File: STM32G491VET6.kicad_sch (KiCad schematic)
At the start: 37 parts, among them CN3 C2839705, CN4 C2839704, J2 TC2030, U2 TYPE-C 16PLT-H10.0, U3 STM32G431CBT6, U9 TCAN3403DRQ1, X1 NX3215SA 32.768KHZ EXS00A-MU0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, X2 NDK NX2016SA-24MHZ-EXS00A-CS1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

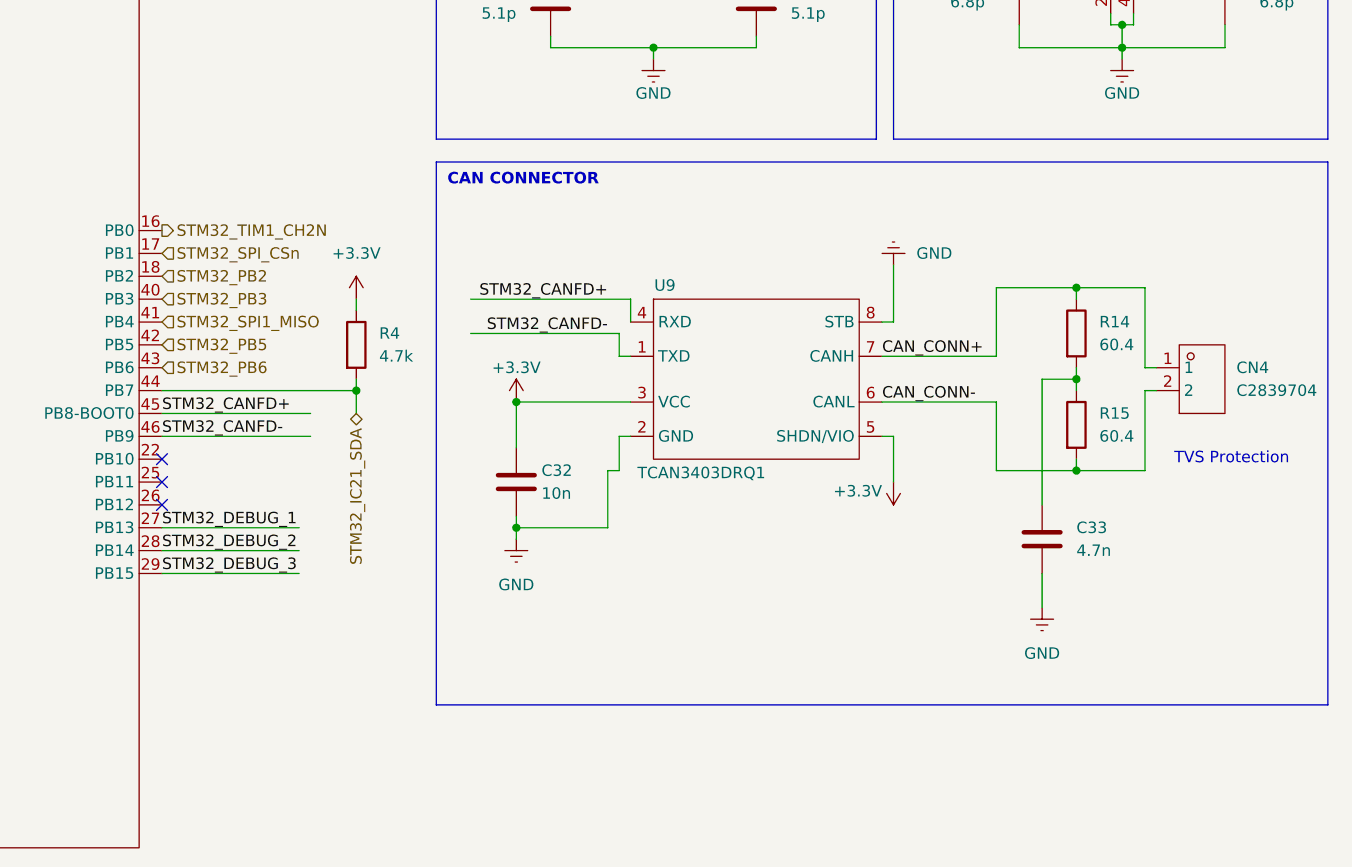
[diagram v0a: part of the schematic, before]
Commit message: update
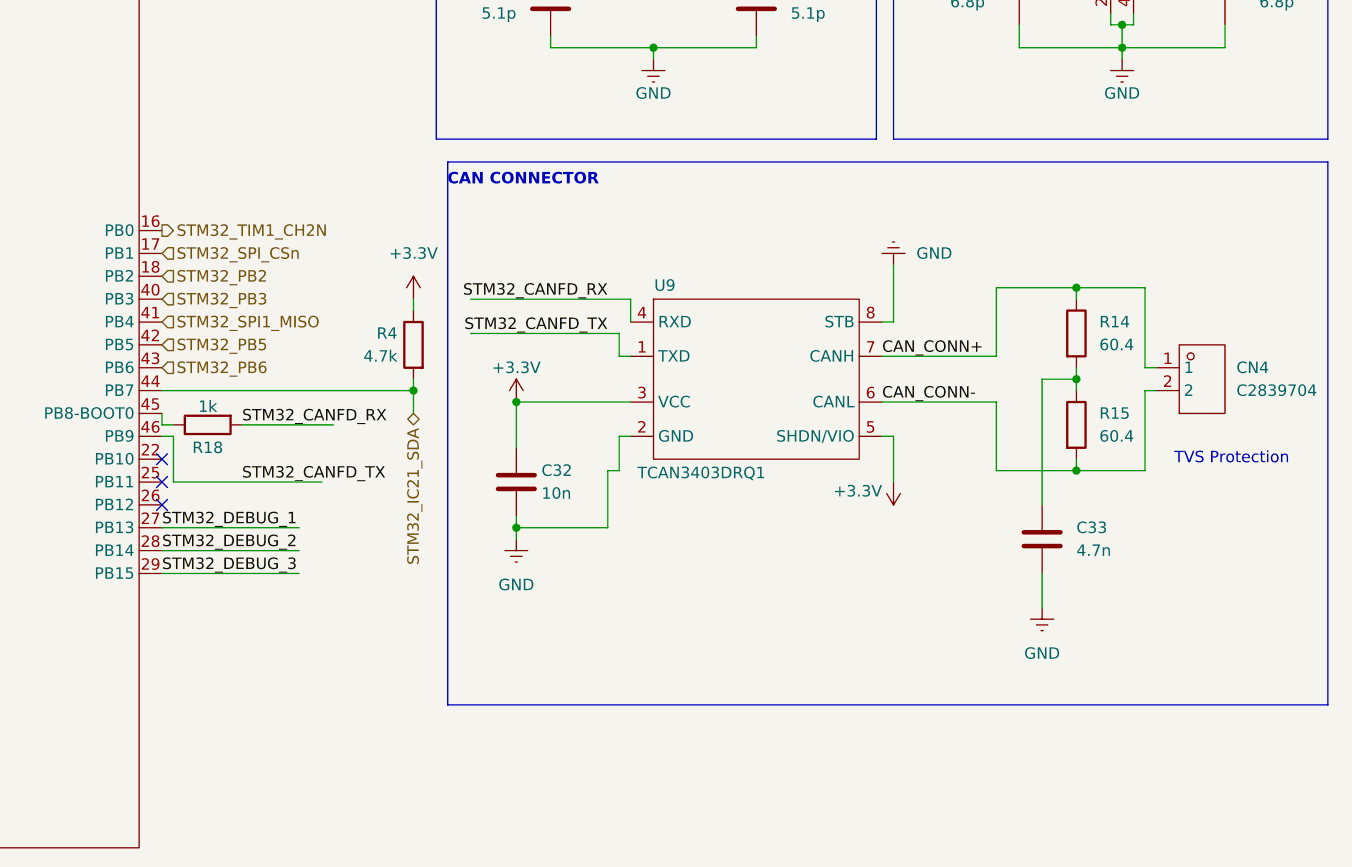
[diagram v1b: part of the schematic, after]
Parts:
- added R18: 1k, PCM_Resistor_SMD_AKL:R_0402_1005Metric, symbol Device:R
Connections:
- net STM32_CANFD+: no longer names the net of U3.45 (PB8-BOOT0)
- net STM32_CANFD+: now also R18.1; no longer U9.4 (RXD)
- net STM32_CANFD- renamed STM32_CANFD_TX
- new net STM32_CANFD_RX: R18.2, U9.4 (RXD)
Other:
- moved on the sheet: R4
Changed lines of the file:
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@@
 	(paper "A4")
 	(rectangle
-		(start 184.15 104.14)
+		(start 185.42 104.14)
 		(end 283.21 164.465)
 		(stroke
@@
 	)
 	(junction
-		(at 175.26 129.54)
+		(at 181.61 129.54)
 		(diameter 0)
 		(color 0 0 0 0)
@@
 	(wire
 		(pts
-			(xy 175.26 119.38) (xy 175.26 120.65)
+			(xy 181.61 119.38) (xy 181.61 120.65)
 		)
 		(stroke
@@
 	(wire
 		(pts
-			(xy 175.26 129.54) (xy 153.67 129.54)
+			(xy 153.67 129.54) (xy 181.61 129.54)
 		)
 		(stroke
@@
 	(wire
 		(pts
-			(xy 185.42 33.02) (xy 185.42 34.29)
+			(xy 153.67 133.35) (xy 153.67 132.08)
 		)
 		(stroke
@@
 	(wire
 		(pts
-			(xy 91.44 165.1) (xy 105.41 165.1)
+			(xy 185.42 33.02) (xy 185.42 34.29)
 		)
 		(stroke
@@
 	(wire
 		(pts
-			(xy 185.42 43.18) (xy 172.72 43.18)
+			(xy 91.44 165.1) (xy 105.41 165.1)
 		)
 		(stroke
@@
 	(wire
 		(pts
-			(xy 153.67 132.08) (xy 170.18 132.08)
+			(xy 185.42 43.18) (xy 172.72 43.18)
 		)
 		(stroke
@@
 	(wire
 		(pts
+			(xy 154.94 139.7) (xy 171.45 139.7)
+		)
+		(stroke
+			(width 0)
+			(type default)
+		)
+	)
+	(wire
+		(pts
 			(xy 20.32 36.83) (xy 20.32 40.64)
 		)
@@
 	(wire
 		(pts
+			(xy 153.67 133.35) (xy 154.94 133.35)
+		)
+		(stroke
+			(width 0)
+			(type default)
+		)
+	)
+	(wire
+		(pts
 			(xy 90.17 160.02) (xy 105.41 160.02)
 		)
@@
 	(wire
 		(pts
-			(xy 175.26 128.27) (xy 175.26 129.54)
+			(xy 181.61 128.27) (xy 181.61 129.54)
 		)
 		(stroke
@@
 	(wire
 		(pts
-			(xy 175.26 129.54) (xy 175.26 132.08)
+			(xy 181.61 129.54) (xy 181.61 132.08)
 		)
 		(stroke
@@
 	(wire
 		(pts
+			(xy 153.67 134.62) (xy 154.94 134.62)
+		)
+		(stroke
+			(width 0)
+			(type default)
+		)
+	)
+	(wire
+		(pts
 			(xy 185.42 33.02) (xy 198.12 33.02)
 		)
@@
 	(wire
 		(pts
+			(xy 162.56 133.35) (xy 172.72 133.35)
+		)
+		(stroke
+			(width 0)
+			(type default)
+		)
+	)
+	(wire
+		(pts
 			(xy 251.46 128.27) (xy 251.46 142.24)
 		)
@@
 	(wire
 		(pts
-			(xy 213.36 80.01) (xy 219.71 80.01)
+			(xy 154.94 134.62) (xy 154.94 139.7)
 		)
 		(stroke
@@
 	(wire
 		(pts
-			(xy 29.21 118.11) (xy 45.72 118.11)
+			(xy 213.36 80.01) (xy 219.71 80.01)
 		)
 		(stroke
@@
 	(wire
 		(pts
-			(xy 104.14 118.11) (xy 105.41 118.11)
+			(xy 29.21 118.11) (xy 45.72 118.11)
 		)
 		(stroke
@@
 	(wire
 		(pts
-			(xy 204.47 134.62) (xy 205.74 134.62)
+			(xy 104.14 118.11) (xy 105.41 118.11)
 		)
 		(stroke
@@
 	(wire
 		(pts
-			(xy 153.67 134.62) (xy 170.18 134.62)
+			(xy 204.47 134.62) (xy 205.74 134.62)
 		)
 		(stroke
@@
 		)
 	)
-	(label "STM32_CANFD+"
+	(label "STM32_CANFD_RX"
 		(at 203.2 119.38 180)
 		(effects
@@
 		)
 	)
-	(label "STM32_CANFD+"
-		(at 153.67 132.08 0)
+	(label "STM32_CANFD_RX"
+		(at 162.56 133.35 0)
 		(effects
 			(font
@@
 		)
 	)
-	(label "STM32_CANFD-"
-		(at 153.67 134.62 0)
+	(label "STM32_CANFD_TX"
+		(at 162.56 139.7 0)
 		(effects
 			(font
@@
 		)
 	)
-	(label "STM32_CANFD-"
+	(label "STM32_CANFD_TX"
 		(at 203.2 123.19 180)
 		(effects
@@
 	(hierarchical_label "STM32_IC21_SDA"
 		(shape bidirectional)
-		(at 175.26 132.08 270)
+		(at 181.61 132.08 270)
 		(effects
 			(font
@@
 	)
 	(symbol
+		(lib_id "Device:R")
+		(at 158.75 133.35 90)
+		(mirror x)
+		(unit 1)
+		(exclude_from_sim no)
+		(in_bom yes)
+		(on_board yes)
+		(dnp no)
+		(property "Reference" "R18"
+			(at 158.75 135.89 90)
+			(effects
+				(font
+					(size 1.27 1.27)
+				)
+			)
+		)
+		(property "Value" "1k"
+			(at 158.75 131.318 90)
+			(effects
+				(font
+					(size 1.27 1.27)
+				)
+			)
+		)
+		(property "Footprint" "PCM_Resistor_SMD_AKL:R_0402_1005Metric"
+			(at 158.75 131.572 90)
+			(effects
+				(font
+					(size 1.27 1.27)
+				)
+				(hide yes)
+			)
+		)
+		(property "Datasheet" "~"
+			(at 158.75 133.35 0)
+			(effects
+				(font
+					(size 1.27 1.27)
+				)
+				(hide yes)
+			)
+		)
+		(property "Description" "Resistor"
+			(at 158.75 133.35 0)
+			(effects
+				(font
+					(size 1.27 1.27)
+				)
+				(hide yes)
+			)
+		)
+		(pin "2"
+		)
+		(pin "1"
+		)
+		(instances
+			(project "foc-stepper-driver"
+				(path "/e8a1091a-f86c-4a0e-9f89-1944d2e62a64/8dccacd0-f830-411d-9fe7-31eb458bafe4"
+					(reference "R18")
+					(unit 1)
+				)
+			)
+		)
+	)
+	(symbol
 		(lib_id "power:+5V")
 		(at 234.95 139.7 0)
@@
 	(symbol
 		(lib_id "power:+3.3V")
-		(at 175.26 119.38 0)
+		(at 181.61 119.38 0)
 		(unit 1)
 		(exclude_from_sim no)
@@
 		(dnp no)
 		(property "Reference" "#PWR037"
-			(at 175.26 123.19 0)
+			(at 181.61 123.19 0)
 			(effects
 				(font
@@
 		)
 		(property "Value" "+3.3V"
-			(at 175.26 114.3 0)
+			(at 181.61 114.3 0)
 			(effects
 				(font
@@
 		)
 		(property "Footprint" ""
-			(at 175.26 119.38 0)
+			(at 181.61 119.38 0)
 			(effects
 				(font
@@
 		)
 		(property "Datasheet" ""
-			(at 175.26 119.38 0)
+			(at 181.61 119.38 0)
 			(effects
 				(font
@@
 		)
 		(property "Description" "Power symbol creates a global label with name \"+3.3V\""
-			(at 175.26 119.38 0)
+			(at 181.61 119.38 0)
 			(effects
 				(font
@@
 	(symbol
 		(lib_id "Device:R")
-		(at 175.26 124.46 0)
+		(at 181.61 124.46 0)
+		(mirror y)
 		(unit 1)
 		(exclude_from_sim no)
@@
 		(on_board yes)
 		(dnp no)
-		(fields_autoplaced yes)
 		(property "Reference" "R4"
-			(at 177.8 123.1899 0)
+			(at 179.832 123.19 0)
 			(effects
 				(font
@@
 		)
 		(property "Value" "4.7k"
-			(at 177.8 125.7299 0)
+			(at 179.832 125.73 0)
 			(effects
 				(font
@@
 		)
 		(property "Footprint" "Capacitor_SMD:C_0201_0603Metric"
-			(at 173.482 124.46 90)
+			(at 183.388 124.46 90)
 			(effects
 				(font
@@
 		)
 		(property "Datasheet" "~"
-			(at 175.26 124.46 0)
+			(at 181.61 124.46 0)
 			(effects
 				(font
@@
 		)
 		(property "Description" "Resistor"
-			(at 175.26 124.46 0)
+			(at 181.61 124.46 0)
 			(effects
 				(font
@@
 		)
 		(property "LCSC" "C25900"
-			(at 177.8 123.1899 0)
+			(at 179.07 123.1899 0)
 			(effects
 				(font
